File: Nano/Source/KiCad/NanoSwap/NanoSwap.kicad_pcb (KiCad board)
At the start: 2 copper layers, 18 parts

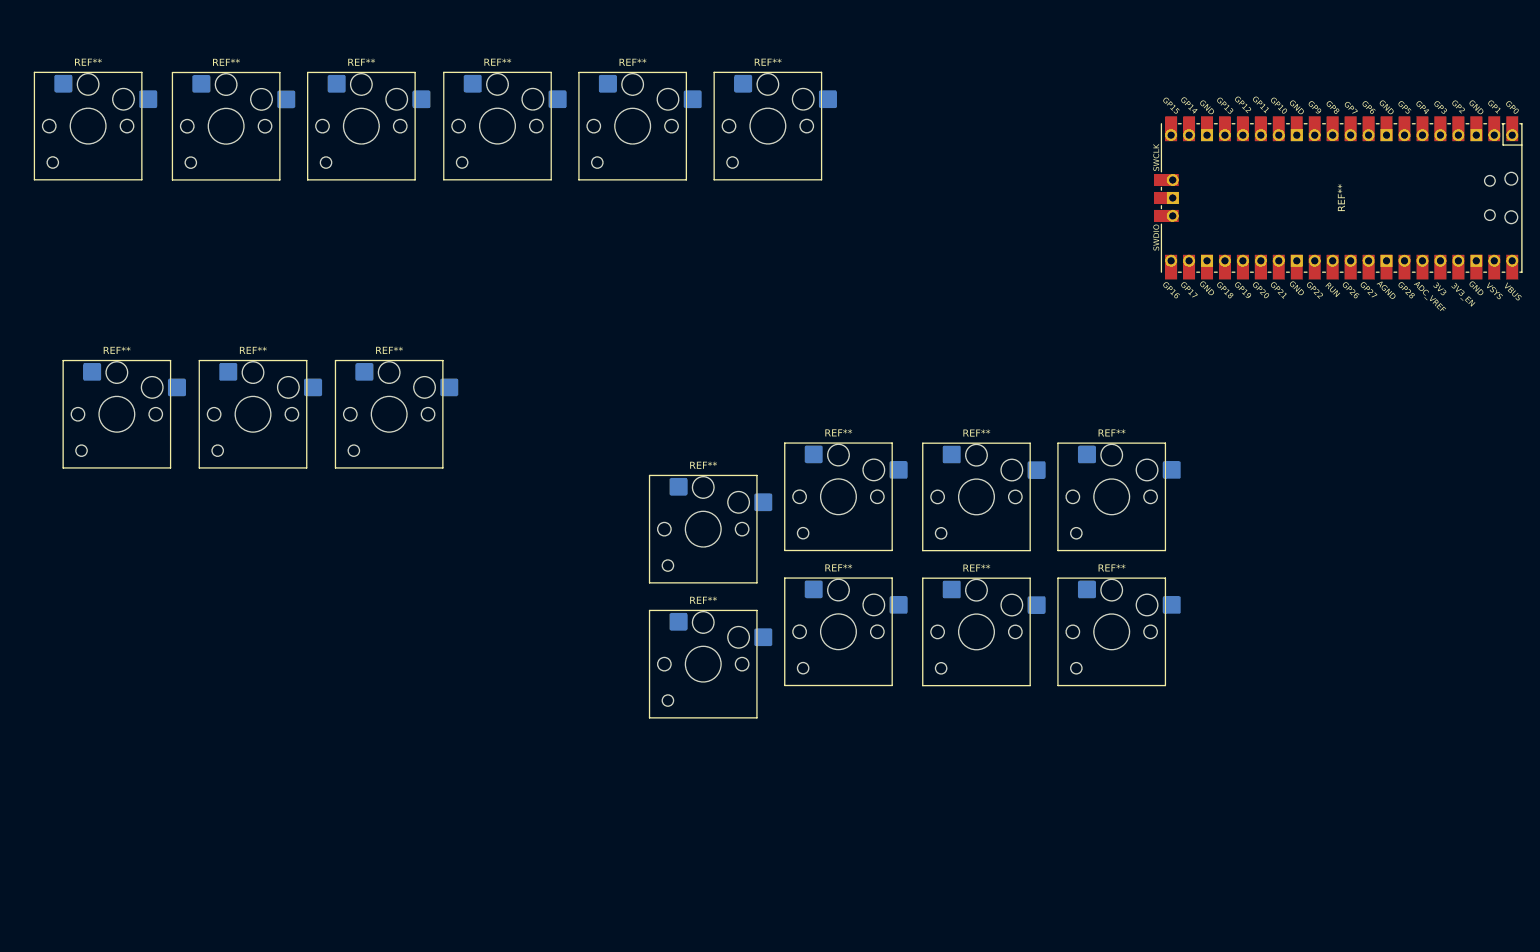
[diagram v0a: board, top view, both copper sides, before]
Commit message: Time for traces
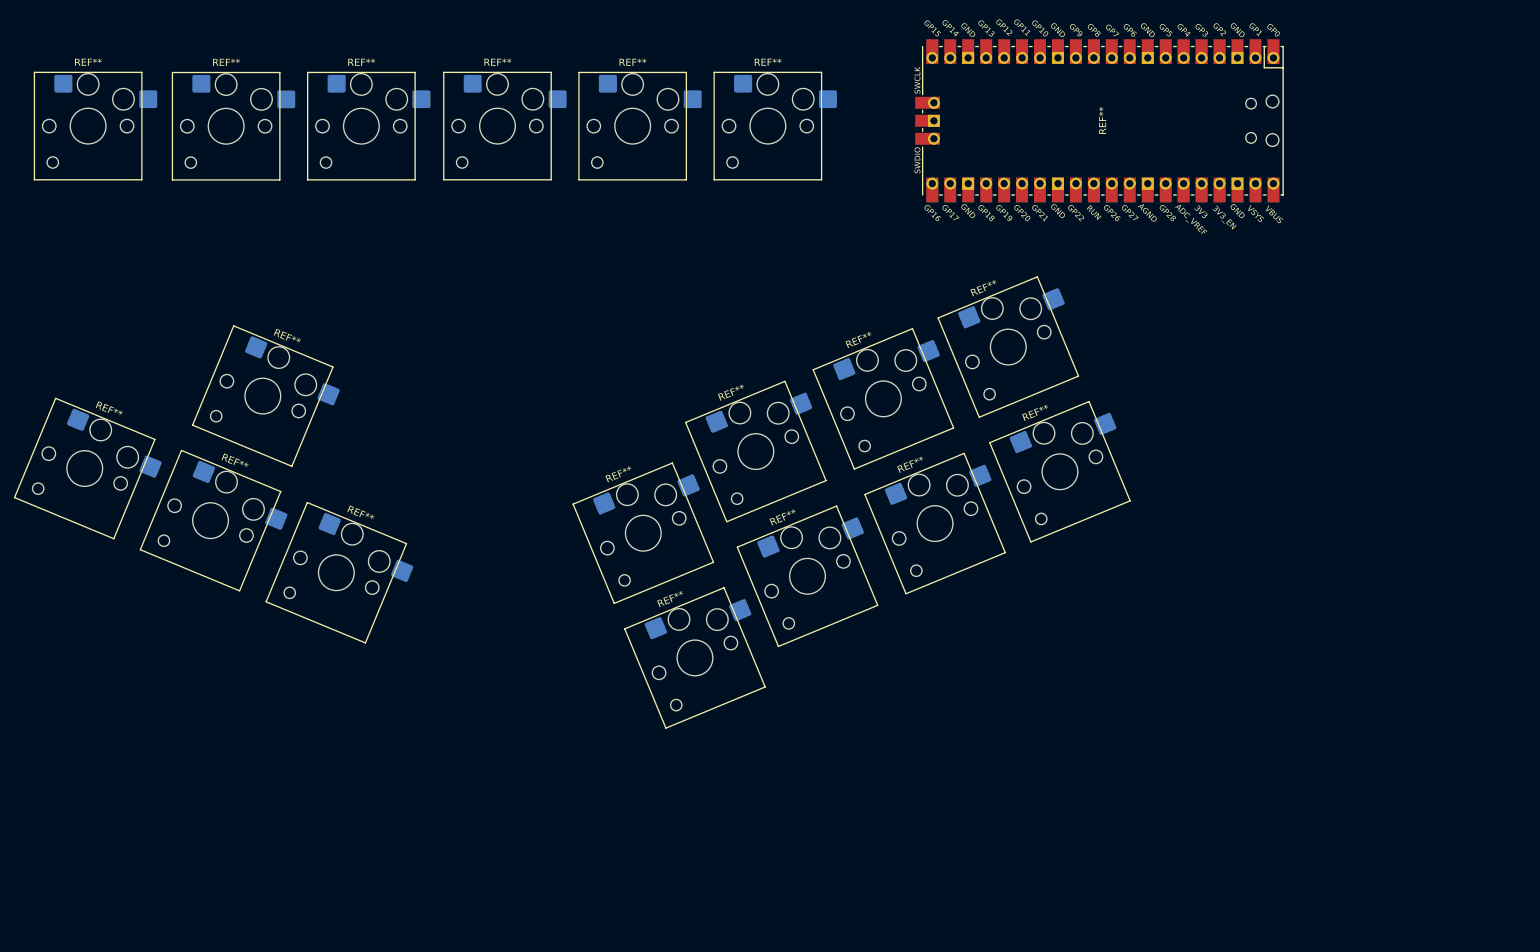
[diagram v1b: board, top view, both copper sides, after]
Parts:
- added REF**: SW_Hotswap_Kailh_Choc_V1V2_1.00u, PCM_Switch_Keyboard_Hotswap_Kailh:SW_Hotswap_Kailh_Choc_V1V2_1.00u, F.Cu at (65.8, 68.7)
- moved REF** 35.5 mm to (184.7, 29.7)
- moved REF** 25.7 mm to (171.3, 61.7), turned to 22.5 degrees
- moved REF** 23.8 mm to (178.6, 79.4), turned to 22.5 degrees
- moved REF** 23.6 mm to (76.2, 93.7), turned to -22.5 degrees
- moved REF** 19.1 mm to (153.6, 69.1), turned to 22.5 degrees
- moved REF** 16.4 mm to (160.9, 86.7), turned to 22.5 degrees
- moved REF** 16.2 mm to (58.4, 86.3), turned to -22.5 degrees
- moved REF** 13.3 mm to (135.6, 76.5), turned to 22.5 degrees
- moved REF** 8.99 mm to (142.9, 94.2), turned to 22.5 degrees
- moved REF** 8.92 mm to (40.6, 78.9), turned to -22.5 degrees
- moved REF** 8.50 mm to (119.6, 88.1), turned to 22.5 degrees
- moved REF** 1.46 mm to (127.0, 105.7), turned to 22.5 degrees

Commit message: Laying down some '''groundwork'''
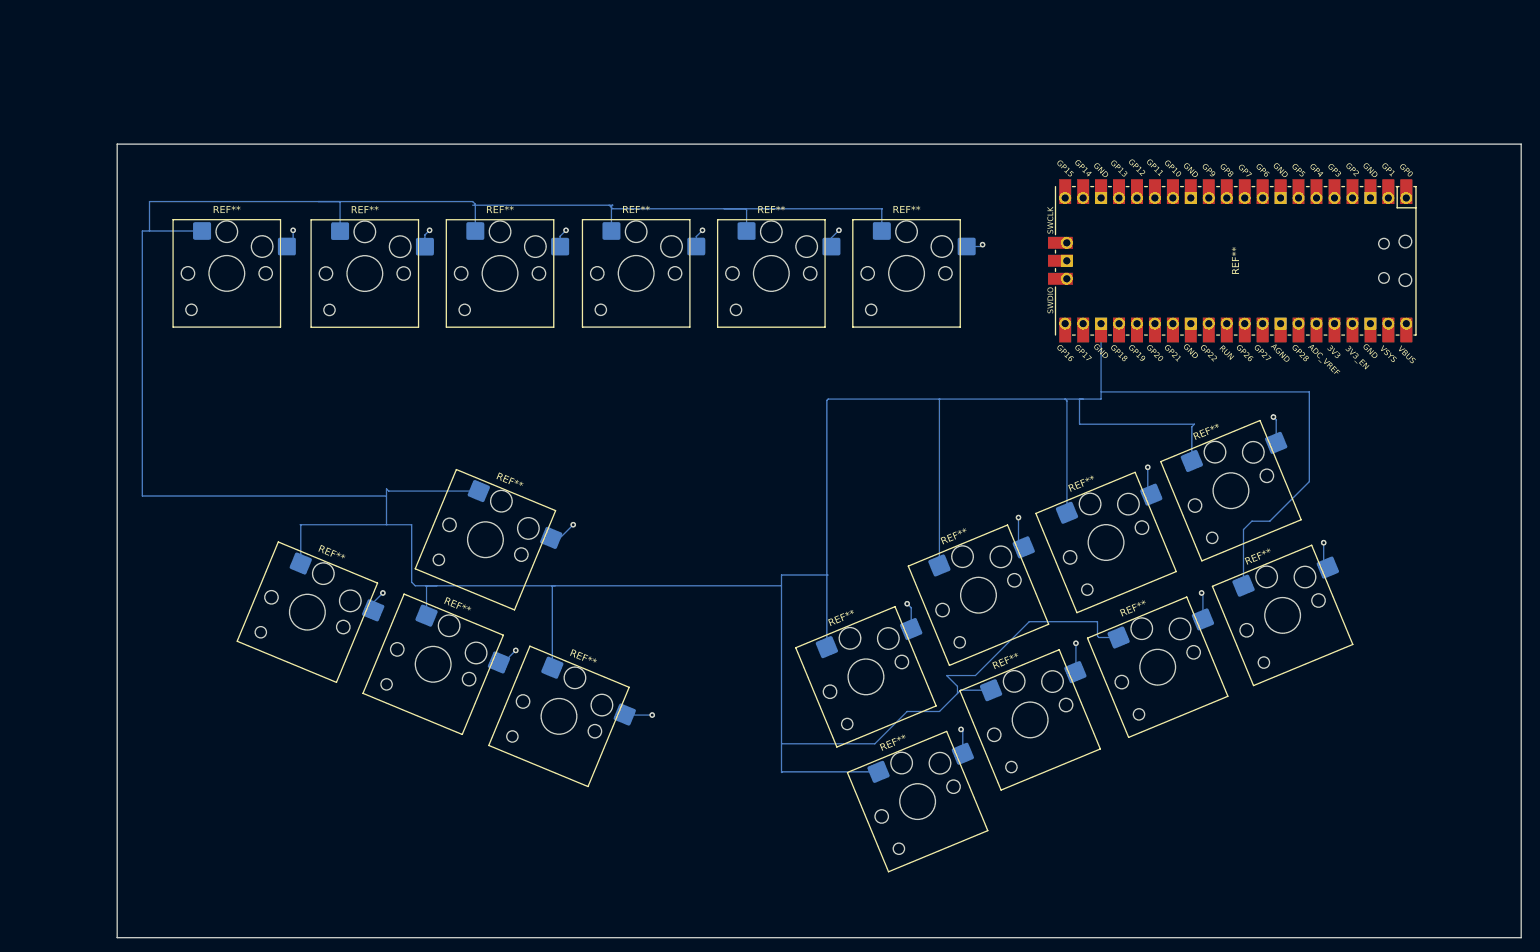
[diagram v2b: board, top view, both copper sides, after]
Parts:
- moved REF** 37.5 mm to (89.9, 106.6)
- moved REF** 37.5 mm to (210.1, 99.7)
- moved REF** 37.5 mm to (72.1, 99.2)
- moved REF** 37.5 mm to (167.1, 96.8)
- moved REF** 37.5 mm to (185.1, 89.4)
- moved REF** 37.5 mm to (151.1, 108.4)
- moved REF** 37.5 mm to (107.7, 114.0)
- moved REF** 37.5 mm to (158.4, 126.0)
- moved REF** 37.5 mm to (97.3, 89.0)
- moved REF** 37.5 mm to (202.8, 82.0)
- moved REF** 37.5 mm to (174.4, 114.5)
- moved REF** 37.5 mm to (192.4, 107.0)
- moved REF** 28.6 mm to (80.2, 51.3)
- moved REF** 28.6 mm to (60.7, 51.3)
- moved REF** 28.6 mm to (118.6, 51.3)
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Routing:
- net (no net): track 0.00 -> 718.9 mm, vias 0 -> 18
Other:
- board outline added: 198.6 x 112.3 mm
